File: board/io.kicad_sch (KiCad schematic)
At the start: 18 parts, among them J2 KEYBOARD, J4 MOUSE, J5 AudioJack3, J9 FTDI serial, U15 LM358, U16 AT89x51xxP, Y2 11.0592MHz

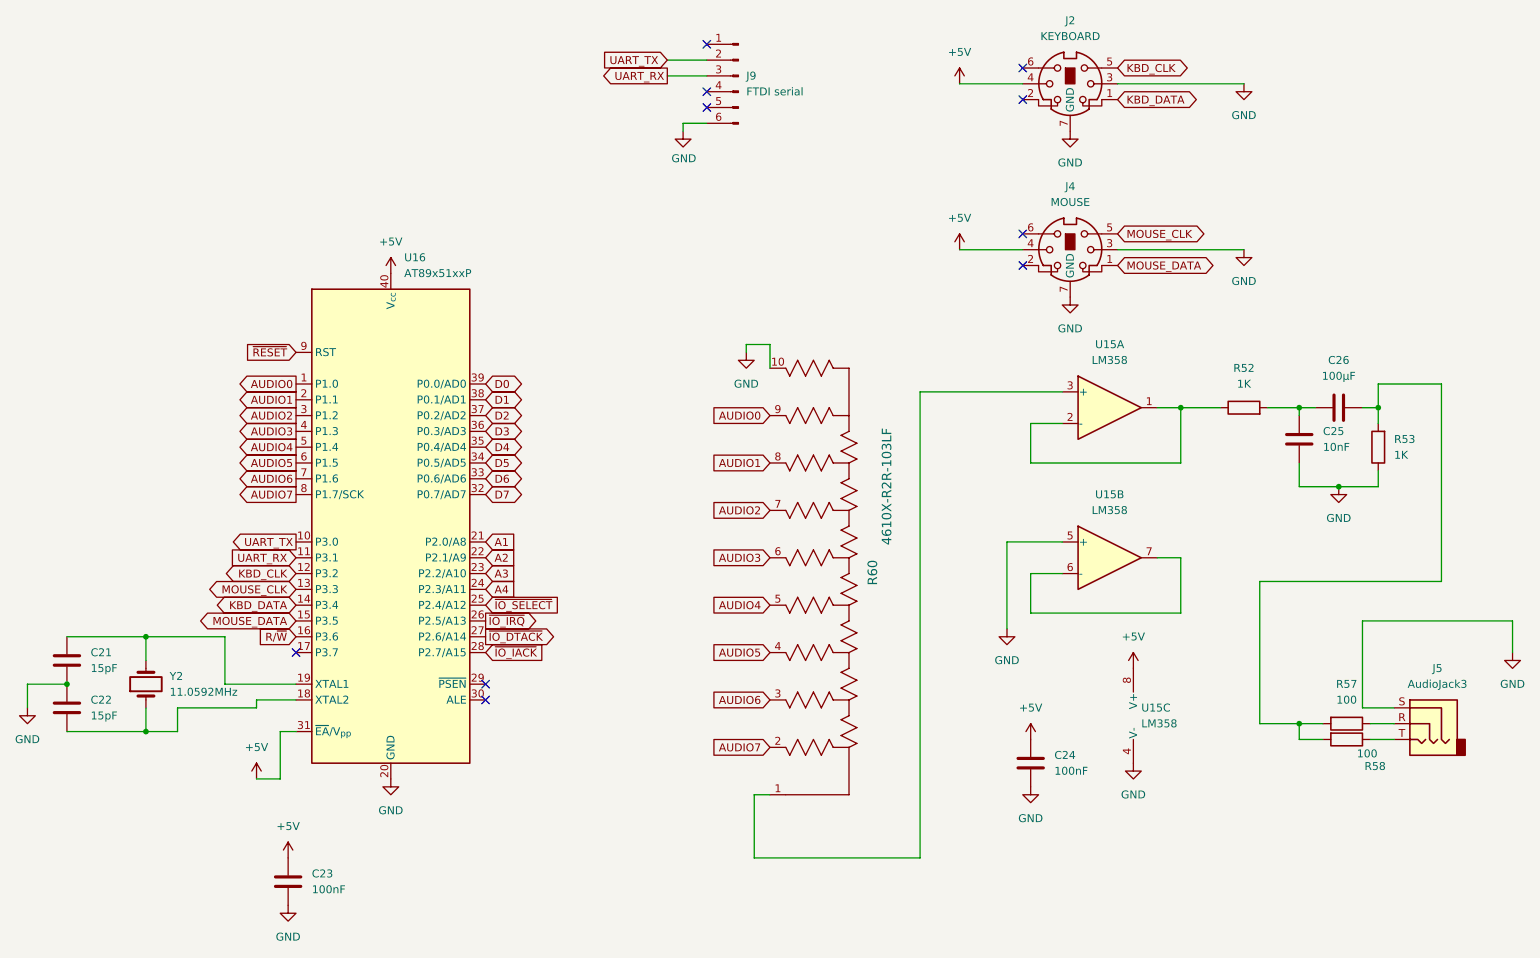
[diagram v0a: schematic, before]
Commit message: checkpoint
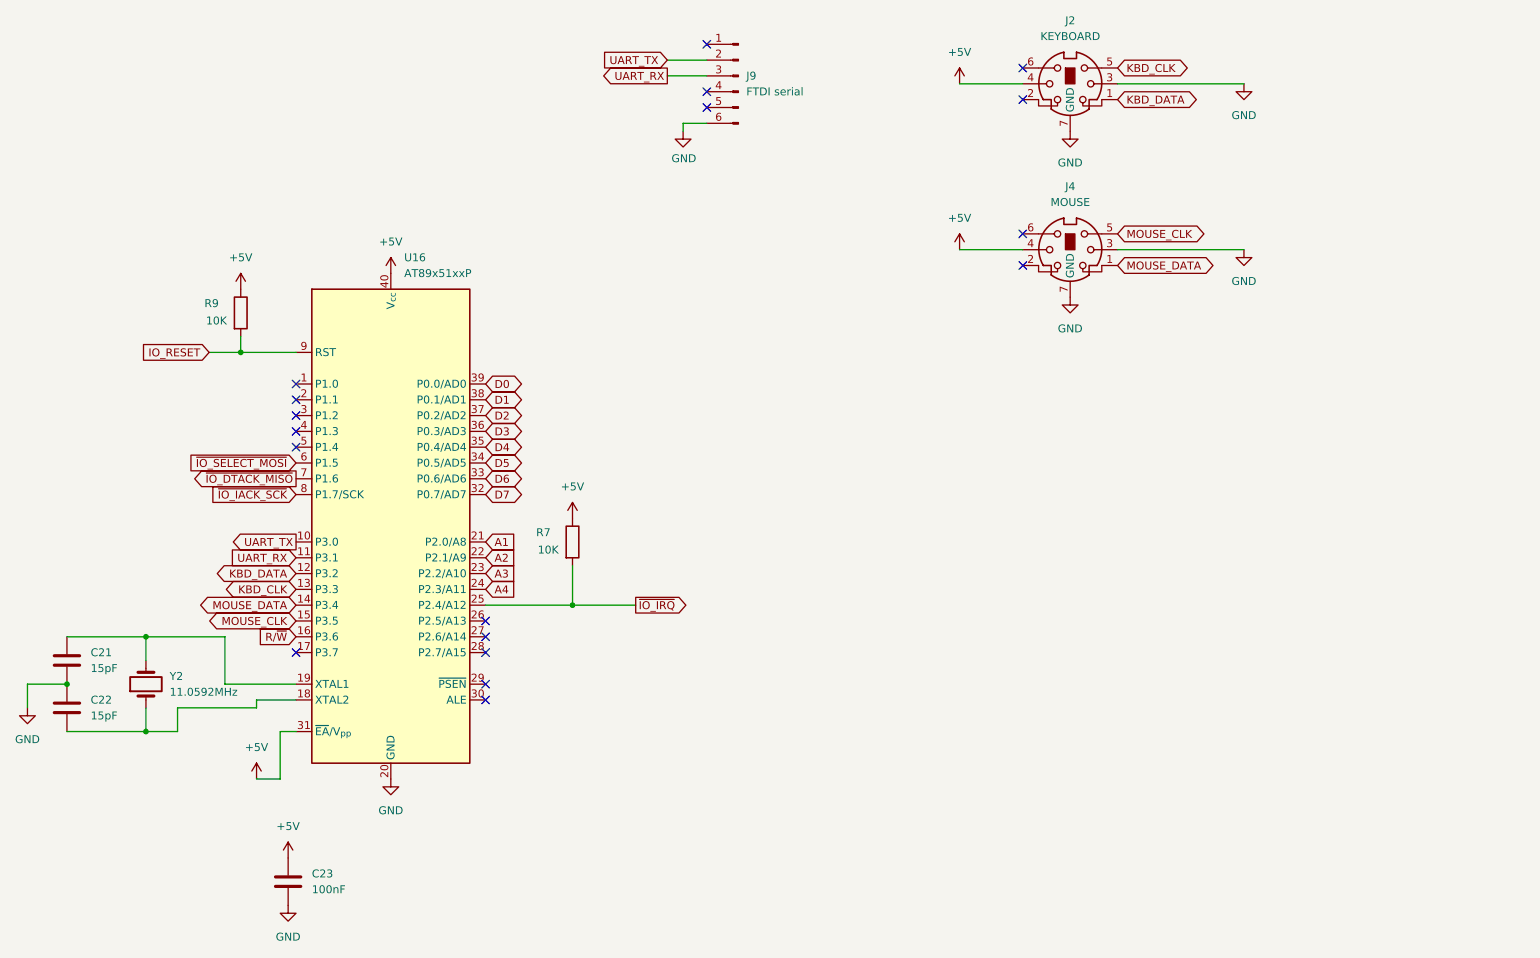
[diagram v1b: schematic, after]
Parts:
- removed C24: 100nF, Capacitor_THT:C_Disc_D5.0mm_W2.5mm_P5.00mm, symbol Device:C
- removed C25: 10nF, Capacitor_THT:C_Disc_D3.0mm_W1.6mm_P2.50mm, symbol Device:C
- removed C26: 100µF, Capacitor_THT:CP_Radial_D5.0mm_P2.50mm, symbol Device:C
- removed J5: AudioJack3, Connector_Audio:Jack_3.5mm_CUI_SJ1-3523N_Horizontal, symbol Connector_Audio:AudioJack3
- removed R52, R53: 1K, Resistor_THT:R_Axial_DIN0207_L6.3mm_D2.5mm_P10.16mm_Horizontal, symbol Device:R
- removed R57, R58: 100, Resistor_THT:R_Axial_DIN0207_L6.3mm_D2.5mm_P10.16mm_Horizontal, symbol Device:R
- removed R60: 4610X-R2R-103LF, board:BO_4610X, symbol 68k_board:4610X-R2R-103LF
- removed U15: LM358, Package_DIP:DIP-8_W7.62mm, symbol Amplifier_Operational:LM358
- added R7, R9: 10K, Resistor_THT:R_Axial_DIN0207_L6.3mm_D2.5mm_P10.16mm_Horizontal, symbol Device:R
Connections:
- net ~{IO_SELECT} is gone; now on net ~{IO_IRQ}: U16.25 (P2.4/A12)
- net +5V: now also R7.1, R9.1
- net KBD_CLK: now also U16.13 (P3.3); no longer U16.12 (P3.2)
- net KBD_DATA: now also U16.12 (P3.2); no longer U16.14 (P3.4)
- net MOUSE_CLK: now also U16.15 (P3.5); no longer U16.13 (P3.3)
- net MOUSE_DATA: now also U16.14 (P3.4); no longer U16.15 (P3.5)
- net ~{IO_IRQ}: now also R7.2; no longer U16.26 (P2.5/A13)
- net AUDIO0: no longer names the net of U16.1 (P1.0)
- net AUDIO1: no longer names the net of U16.2 (P1.1)
- net AUDIO2: no longer names the net of U16.3 (P1.2)
- net AUDIO3: no longer names the net of U16.4 (P1.3)
- net AUDIO4: no longer names the net of U16.5 (P1.4)
- net AUDIO5 renamed ~{IO_SELECT_MOSI}
- net AUDIO6 renamed ~{IO_DTACK_MISO}
- net AUDIO7 renamed ~{IO_IACK_SCK}
- net ~{IO_DTACK}: no longer names the net of U16.27 (P2.6/A14)
- net ~{IO_IACK}: no longer names the net of U16.28 (P2.7/A15)
- net ~{RESET} renamed IO_RESET
- net IO_RESET: now also R9.2
- no-connect marks 10 -> 18

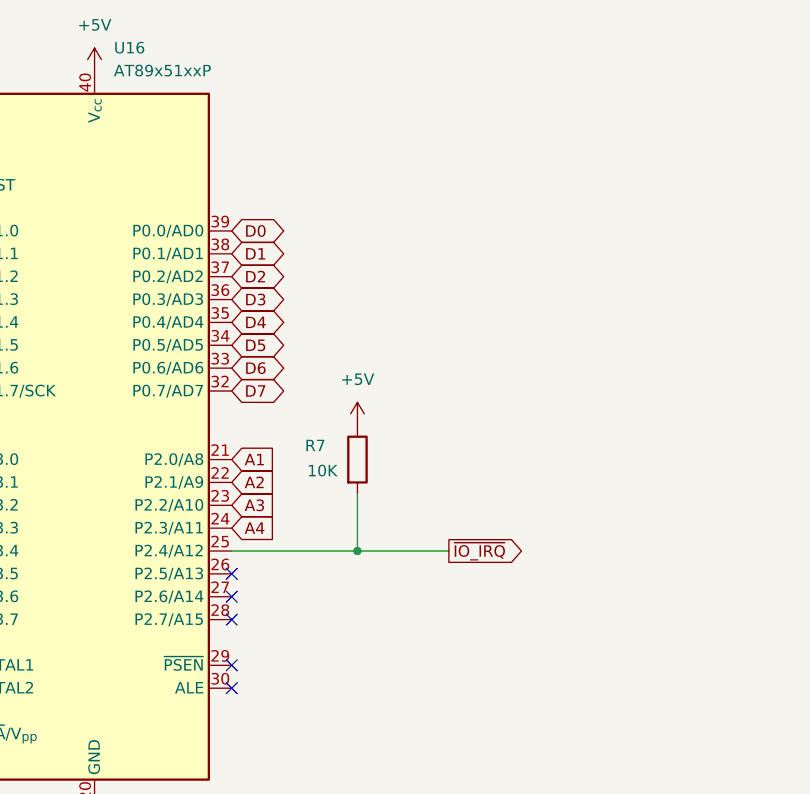
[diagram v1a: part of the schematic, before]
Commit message: Board rev1 PCB complete, already have a spot fix
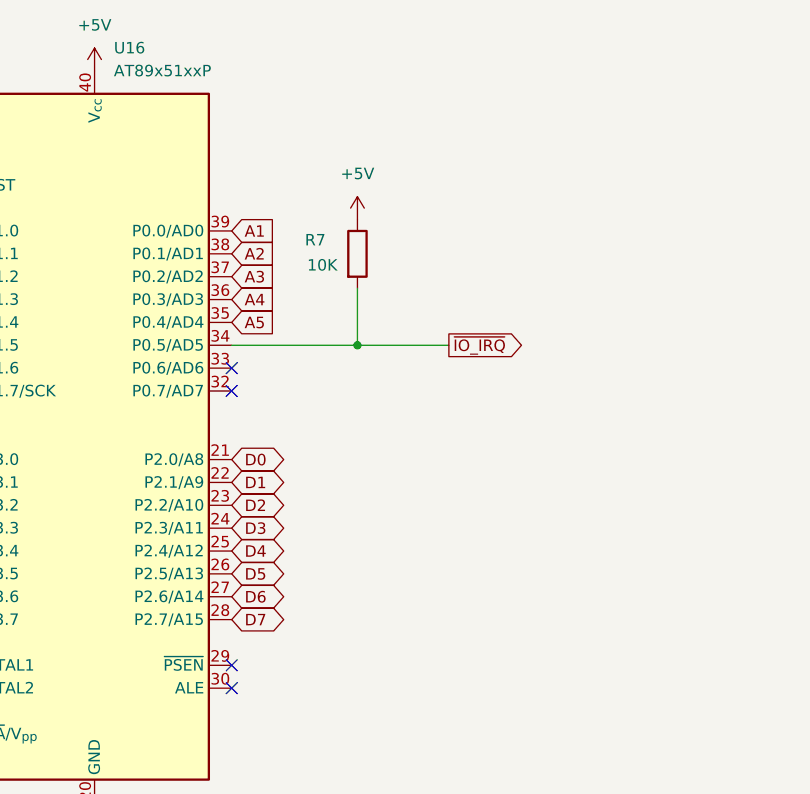
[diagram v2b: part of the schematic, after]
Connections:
- net A1: now also U16.39 (P0.0/AD0); no longer U16.21 (P2.0/A8)
- net A2: now also U16.38 (P0.1/AD1); no longer U16.22 (P2.1/A9)
- net A3: now also U16.37 (P0.2/AD2); no longer U16.23 (P2.2/A10)
- net A4: now also U16.36 (P0.3/AD3); no longer U16.24 (P2.3/A11)
- net D0: now also U16.21 (P2.0/A8); no longer U16.39 (P0.0/AD0)
- net D1: now also U16.22 (P2.1/A9); no longer U16.38 (P0.1/AD1)
- net D2: now also U16.23 (P2.2/A10); no longer U16.37 (P0.2/AD2)
- net D3: now also U16.24 (P2.3/A11); no longer U16.36 (P0.3/AD3)
- net D4: now also U16.25 (P2.4/A12); no longer U16.35 (P0.4/AD4)
- net D5: now also U16.26 (P2.5/A13); no longer U16.34 (P0.5/AD5)
- net D6: now also U16.27 (P2.6/A14); no longer U16.33 (P0.6/AD6)
- net D7: now also U16.28 (P2.7/A15); no longer U16.32 (P0.7/AD7)
- net ~{IO_IRQ}: now also U16.34 (P0.5/AD5); no longer U16.25 (P2.4/A12)
- new net A5: U16.35 (P0.4/AD4)
- no-connect marks 18 -> 17
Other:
- moved on the sheet: R7
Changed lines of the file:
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@@
 	(paper "USLetter")
 	(junction
-		(at 104.14 113.03)
+		(at 104.14 90.17)
 		(diameter 0)
 		(color 0 0 0 0)
@@
 	)
 	(no_connect
-		(at 90.17 120.65)
+		(at 90.17 95.25)
 	)
 	(no_connect
@@
 	)
 	(no_connect
-		(at 90.17 115.57)
-	)
-	(no_connect
 		(at 59.69 80.01)
 	)
@@
 	)
 	(no_connect
-		(at 90.17 118.11)
+		(at 90.17 92.71)
 	)
 	(no_connect
@@
 	(wire
 		(pts
-			(xy 114.3 113.03) (xy 104.14 113.03)
+			(xy 114.3 90.17) (xy 104.14 90.17)
 		)
 		(stroke
@@
 	(wire
 		(pts
-			(xy 104.14 113.03) (xy 90.17 113.03)
+			(xy 104.14 90.17) (xy 90.17 90.17)
 		)
 		(stroke
@@
 	(wire
 		(pts
-			(xy 104.14 106.68) (xy 104.14 113.03)
+			(xy 104.14 83.82) (xy 104.14 90.17)
 		)
 		(stroke
@@
 	(global_label "A1"
 		(shape input)
-		(at 90.17 102.87 0)
+		(at 90.17 77.47 0)
 		(fields_autoplaced yes)
 		(effects
@@
 		)
 		(property "Intersheetrefs" "${INTERSHEET_REFS}"
-			(at 95.4533 102.87 0)
+			(at 95.4533 77.47 0)
 			(effects
 				(font
@@
 	(global_label "D0"
 		(shape tri_state)
-		(at 90.17 77.47 0)
+		(at 90.17 102.87 0)
 		(fields_autoplaced yes)
 		(effects
@@
 		)
 		(property "Intersheetrefs" "${INTERSHEET_REFS}"
-			(at 96.746 77.47 0)
+			(at 96.746 102.87 0)
 			(effects
 				(font
@@
 	(global_label "D2"
 		(shape tri_state)
-		(at 90.17 82.55 0)
+		(at 90.17 107.95 0)
 		(fields_autoplaced yes)
 		(effects
@@
 		)
 		(property "Intersheetrefs" "${INTERSHEET_REFS}"
-			(at 96.746 82.55 0)
+			(at 96.746 107.95 0)
 			(effects
 				(font
@@
 	(global_label "~{IO_IRQ}"
 		(shape output)
-		(at 114.3 113.03 0)
+		(at 114.3 90.17 0)
 		(fields_autoplaced yes)
 		(effects
@@
 		)
 		(property "Intersheetrefs" "${INTERSHEET_REFS}"
-			(at 123.3934 113.03 0)
+			(at 123.3934 90.17 0)
 			(effects
 				(font
@@
 	(global_label "D5"
 		(shape tri_state)
-		(at 90.17 90.17 0)
+		(at 90.17 115.57 0)
 		(fields_autoplaced yes)
 		(effects
@@
 		)
 		(property "Intersheetrefs" "${INTERSHEET_REFS}"
-			(at 96.746 90.17 0)
+			(at 96.746 115.57 0)
+			(effects
+				(font
+					(size 1.27 1.27)
+				)
+				(justify left)
+				(hide yes)
+			)
+		)
+	)
+	(global_label "A5"
+		(shape input)
+		(at 90.17 87.63 0)
+		(fields_autoplaced yes)
+		(effects
+			(font
+				(size 1.27 1.27)
+			)
+			(justify left)
+		)
+		(property "Intersheetrefs" "${INTERSHEET_REFS}"
+			(at 95.4533 87.63 0)
 			(effects
 				(font
@@
 	(global_label "D6"
 		(shape tri_state)
-		(at 90.17 92.71 0)
+		(at 90.17 118.11 0)
 		(fields_autoplaced yes)
 		(effects
@@
 		)
 		(property "Intersheetrefs" "${INTERSHEET_REFS}"
-			(at 96.746 92.71 0)
+			(at 96.746 118.11 0)
 			(effects
 				(font
@@
 	(global_label "D1"
 		(shape tri_state)
-		(at 90.17 80.01 0)
+		(at 90.17 105.41 0)
 		(fields_autoplaced yes)
 		(effects
@@
 		)
 		(property "Intersheetrefs" "${INTERSHEET_REFS}"
-			(at 96.746 80.01 0)
+			(at 96.746 105.41 0)
 			(effects
 				(font
@@
 	(global_label "A3"
 		(shape input)
-		(at 90.17 107.95 0)
+		(at 90.17 82.55 0)
 		(fields_autoplaced yes)
 		(effects
@@
 		)
 		(property "Intersheetrefs" "${INTERSHEET_REFS}"
-			(at 95.4533 107.95 0)
+			(at 95.4533 82.55 0)
 			(effects
 				(font
@@
 	(global_label "D3"
 		(shape tri_state)
-		(at 90.17 85.09 0)
+		(at 90.17 110.49 0)
 		(fields_autoplaced yes)
 		(effects
@@
 		)
 		(property "Intersheetrefs" "${INTERSHEET_REFS}"
-			(at 96.746 85.09 0)
+			(at 96.746 110.49 0)
 			(effects
 				(font
@@
 	(global_label "D4"
 		(shape tri_state)
-		(at 90.17 87.63 0)
+		(at 90.17 113.03 0)
 		(fields_autoplaced yes)
 		(effects
@@
 		)
 		(property "Intersheetrefs" "${INTERSHEET_REFS}"
-			(at 96.746 87.63 0)
+			(at 96.746 113.03 0)
 			(effects
 				(font
@@
 	(global_label "A4"
 		(shape input)
-		(at 90.17 110.49 0)
+		(at 90.17 85.09 0)
 		(fields_autoplaced yes)
 		(effects
@@
 		)
 		(property "Intersheetrefs" "${INTERSHEET_REFS}"
-			(at 95.4533 110.49 0)
+			(at 95.4533 85.09 0)
 			(effects
 				(font
@@
 	(global_label "D7"
 		(shape tri_state)
-		(at 90.17 95.25 0)
+		(at 90.17 120.65 0)
 		(fields_autoplaced yes)
 		(effects
@@
 		)
 		(property "Intersheetrefs" "${INTERSHEET_REFS}"
-			(at 96.746 95.25 0)
+			(at 96.746 120.65 0)
 			(effects
 				(font
@@
 	(global_label "A2"
 		(shape input)
-		(at 90.17 105.41 0)
+		(at 90.17 80.01 0)
 		(fields_autoplaced yes)
 		(effects
@@
 		)
 		(property "Intersheetrefs" "${INTERSHEET_REFS}"
-			(at 95.4533 105.41 0)
+			(at 95.4533 80.01 0)
 			(effects
 				(font
@@
 	(symbol
 		(lib_id "Device:R")
-		(at 104.14 102.87 0)
+		(at 104.14 80.01 0)
 		(unit 1)
 		(exclude_from_sim no)
@@
 		(dnp no)
 		(property "Reference" "R7"
-			(at 98.298 101.346 0)
+			(at 98.298 78.486 0)
 			(effects
 				(font
@@
 		)
 		(property "Value" "10K"
-			(at 98.552 104.14 0)
+			(at 98.552 81.28 0)
 			(effects
 				(font
@@
 		)
 		(property "Footprint" "Resistor_THT:R_Axial_DIN0207_L6.3mm_D2.5mm_P10.16mm_Horizontal"
-			(at 102.362 102.87 90)
+			(at 102.362 80.01 90)
 			(effects
 				(font
@@
 		)
 		(property "Datasheet" "~"
-			(at 104.14 102.87 0)
+			(at 104.14 80.01 0)
 			(effects
 				(font
@@
 		)
 		(property "Description" "Resistor"
-			(at 104.14 102.87 0)
+			(at 104.14 80.01 0)
 			(effects
 				(font
@@
 	(symbol
 		(lib_id "power:+5V")
-		(at 104.14 99.06 0)
+		(at 104.14 76.2 0)
 		(unit 1)
 		(exclude_from_sim no)
@@
 		(fields_autoplaced yes)
 		(property "Reference" "#PWR082"
-			(at 104.14 102.87 0)
+			(at 104.14 80.01 0)
 			(effects
 				(font
@@
 		)
 		(property "Value" "+5V"
-			(at 104.14 93.98 0)
+			(at 104.14 71.12 0)
 			(effects
 				(font
@@
 		)
 		(property "Footprint" ""
-			(at 104.14 99.06 0)
+			(at 104.14 76.2 0)
 			(effects
 				(font
@@
 		)
 		(property "Datasheet" ""
-			(at 104.14 99.06 0)
+			(at 104.14 76.2 0)
 			(effects
 				(font
@@
 		)
 		(property "Description" "Power symbol creates a global label with name \"+5V\""
-			(at 104.14 99.06 0)
-			(effects
-				(font
+			(at 104.14 76.2 0)
+			(effects
+				(font
